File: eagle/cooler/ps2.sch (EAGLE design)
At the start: 8 parts, among them J1 PIN2F061.100, J2 PIN2F061.100, J3 PIN2F061.100, J4 PIN2F061.100, J5 PIN2F061.100, J6 PIN2F061.100

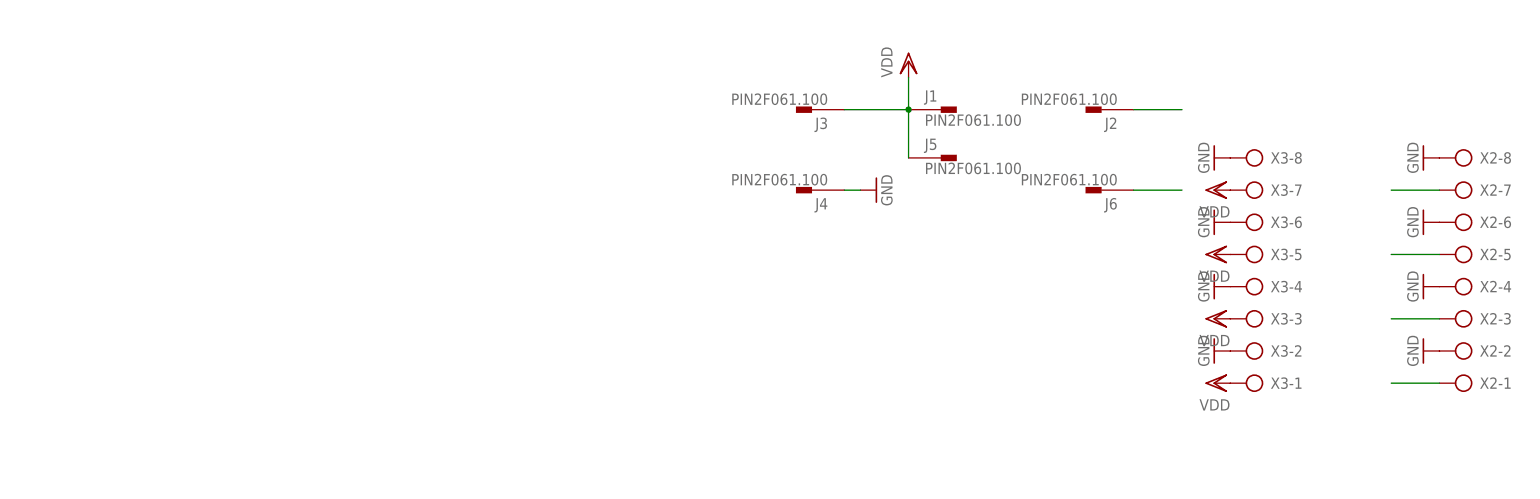
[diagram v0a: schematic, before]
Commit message: layouts
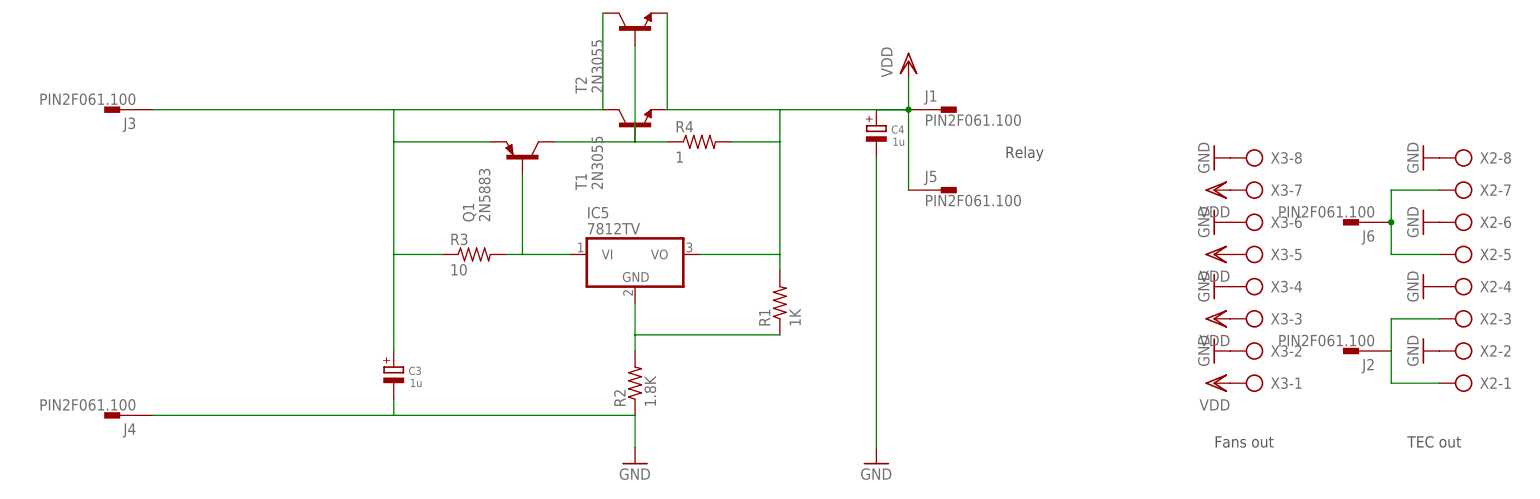
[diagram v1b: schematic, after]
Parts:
- added C3, C4: 1u, rcl:CPOL-EUE10-20
- added IC5: 7812TV, linear:7812TV
- added Q1: 2N5883, transistor-pnp:2N4905
- added R1: 1K, rcl:R-US_0207/15
- added R2: 1.8K, rcl:R-US_0207/15
- added R3: 10, rcl:R-US_0207/15
- added R4: 1, rcl:R-US_0922/22
- added T1, T2: 2N3055, transistor:2N3055
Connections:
- new net N$1: Q1.C, R4.1, T1.B, T2.B
- new net N$4: IC5.VI, Q1.B, R3.2
- new net N$5: IC5.GND, R1.1, R2.2
- new net VIN: C3.+, J3.1, Q1.E, R3.1, T1.C, T2.C
- net GND: now also C3.-, C4.-, R2.1
- net TEC1: now also X2-1.KL, X2-3.KL
- net TEC2: now also X2-5.KL
- net VDD: now also C4.+, IC5.VO, R1.2, R4.2, T1.E, T2.E; no longer J3.1
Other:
- note added: "Fans out"
- note added: "Relay"
- note added: "TEC out"
- moved on the sheet: J2, J3, J4, J5, J6
